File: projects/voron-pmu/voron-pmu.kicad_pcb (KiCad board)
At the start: 2 copper layers, 131 x 64.5 mm, 13 parts, among them J1 Critical loads, J2 Non-critical loads, J3 Critical supply, J4 Non-critical supply, J5 Pwr-loss-1, J6 Pwr-loss-2, K1 FINDER-40.52, K2 FINDER-40.52, K3 FINDER-40.52, K4 FINDER-40.52, SW1 SW_Push, SW2 SW_Push_Open

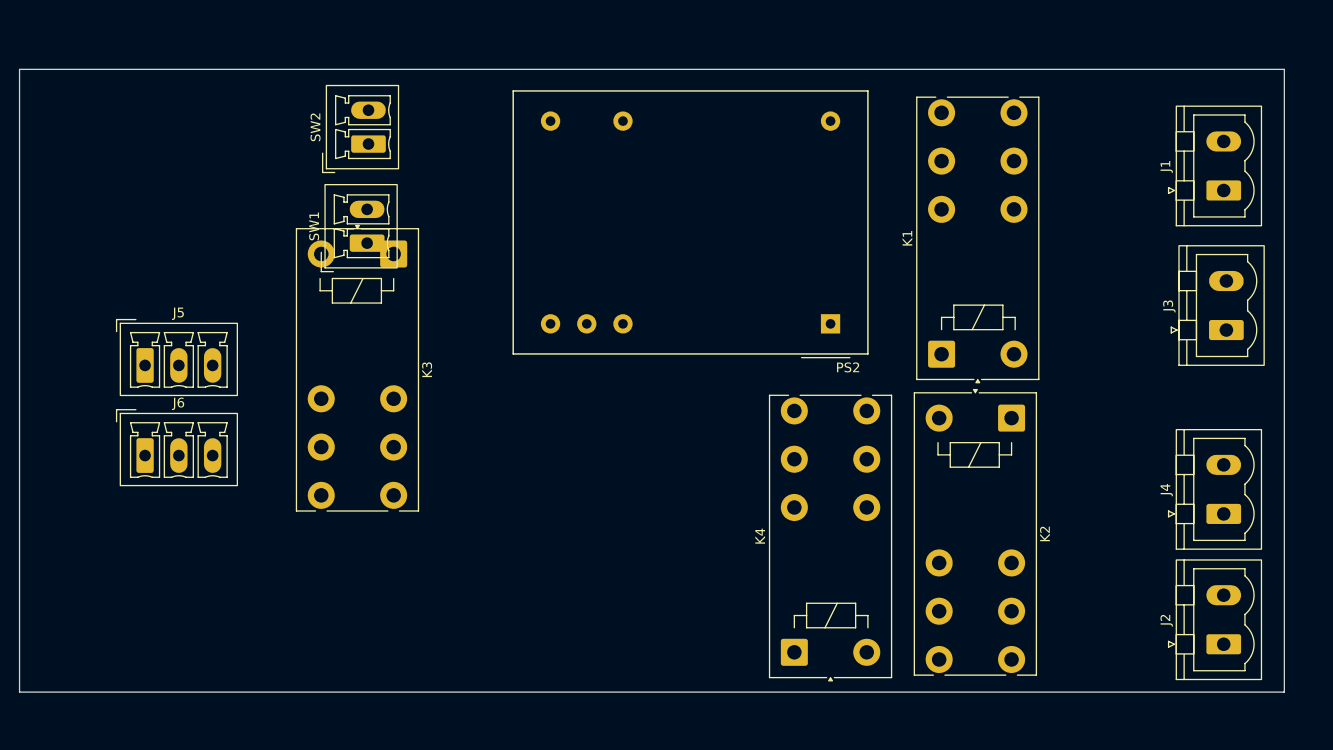
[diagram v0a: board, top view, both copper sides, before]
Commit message: Re-saving.
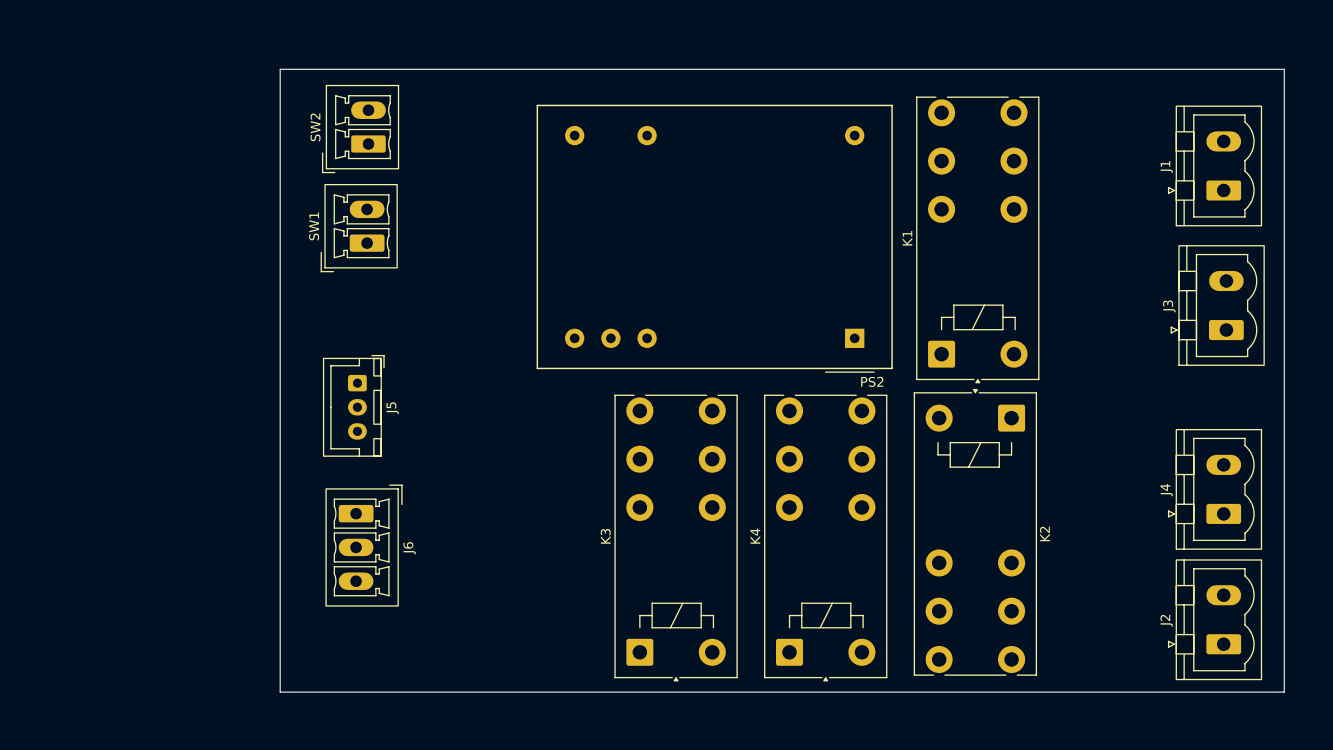
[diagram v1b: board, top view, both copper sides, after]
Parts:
- J5: footprint Connector_Phoenix_MC:PhoenixContact_MCV_1,5_3-G-3.5_1x03_P3.50mm_Vertical -> Connector_JST:JST_XH_B3B-XH-A_1x03_P2.50mm_Vertical
- moved K3 48.5 mm to (133.8, 110.4), turned to 90 degrees
- moved J6 22.7 mm to (104.4, 96.0), turned to -90 degrees
- moved J5 22.1 mm to (104.5, 82.5), turned to -90 degrees
- moved PS2 2.92 mm to (156.0, 77.9)
- moved K4 0.50 mm to (149.2, 110.4)
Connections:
- PS2 pad 5: unconnected-(PS2-AC(L)-Pad5) -> Net-(J3-Pin_1)
- PS2 pad 6: unconnected-(PS2-AC(N)-Pad6) -> Net-(J3-Pin_2)
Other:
- board size 131 x 64.5 mm -> 104 x 64.5 mm

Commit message: Prettyfing schematics.
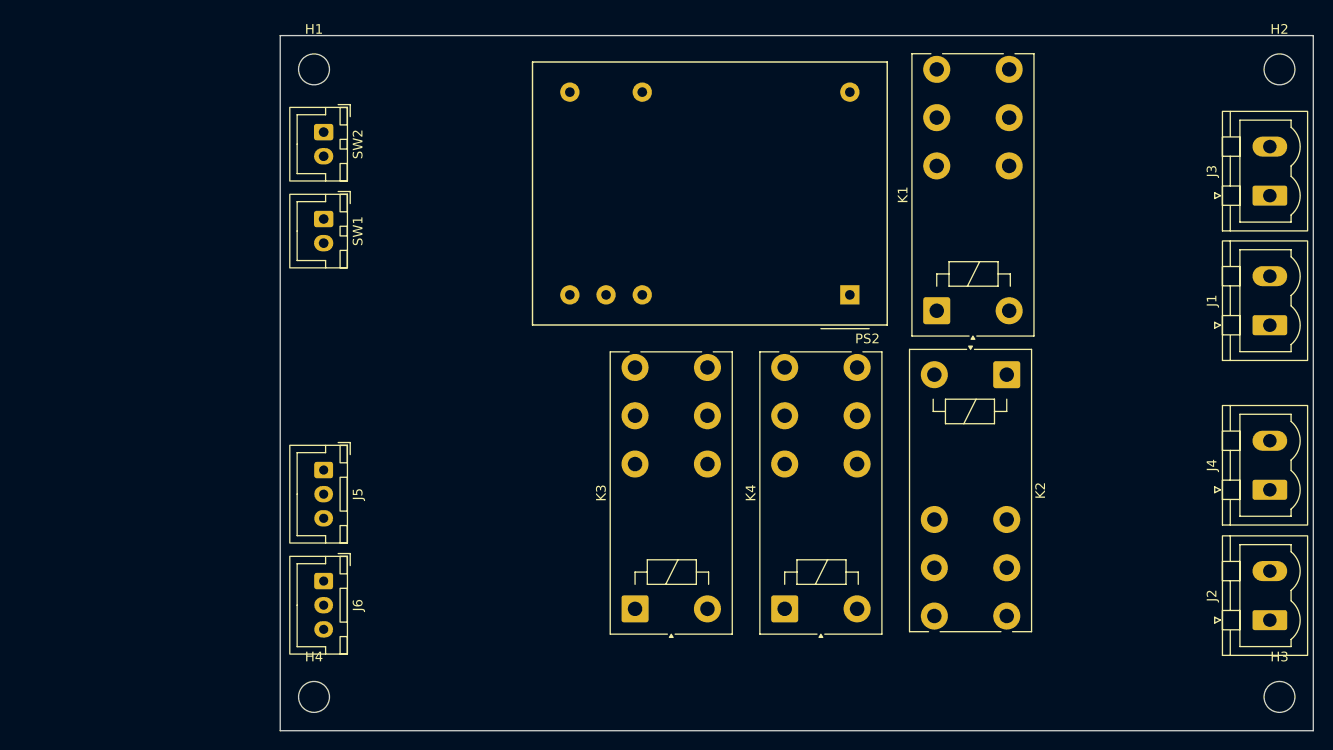
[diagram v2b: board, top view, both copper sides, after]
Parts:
- added H1: MountingHole, MountingHole:MountingHole_3.2mm_M3, F.Cu at (100.0, 50.0)
- added H2: MountingHole, MountingHole:MountingHole_3.2mm_M3, F.Cu at (200.0, 50.0)
- added H3: MountingHole, MountingHole:MountingHole_3.2mm_M3, F.Cu at (200.0, 115.0)
- added H4: MountingHole, MountingHole:MountingHole_3.2mm_M3, F.Cu at (100.0, 115.0)
- J6: footprint Connector_Phoenix_MC:PhoenixContact_MCV_1,5_3-G-3.5_1x03_P3.50mm_Vertical -> Connector_JST:JST_XH_B3B-XH-A_1x03_P2.50mm_Vertical
- SW1: value SW_Push -> sw-on; footprint Connector_Phoenix_MC:PhoenixContact_MCV_1,5_2-G-3.5_1x02_P3.50mm_Vertical -> Connector_JST:JST_XH_B2B-XH-A_1x02_P2.50mm_Vertical
- SW2: value SW_Push_Open -> sw-off; footprint Connector_Phoenix_MC:PhoenixContact_MCV_1,5_2-G-3.5_1x02_P3.50mm_Vertical -> Connector_JST:JST_XH_B2B-XH-A_1x02_P2.50mm_Vertical
- moved J1 14.8 mm to (199.0, 76.5)
- moved J3 14.6 mm to (199.0, 63.1)
- moved J5 9.66 mm to (101.0, 91.5)
- moved J6 7.75 mm to (101.0, 103.0)
- moved J2 5.39 mm to (199.0, 107.0)
- moved J4 5.39 mm to (199.0, 93.5)
- moved SW1 5.15 mm to (101.0, 65.5), turned to -90 degrees
- moved SW2 4.80 mm to (101.0, 56.5), turned to -90 degrees
- moved K1 4.53 mm to (164.5, 75.0)
- moved K2 4.53 mm to (171.8, 81.6)
- moved K3 4.53 mm to (133.2, 105.9)
- moved K4 4.53 mm to (148.8, 105.9)
- moved PS2 4.53 mm to (155.5, 73.4)
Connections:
- net power-good renamed +24V-sw
- PS2 pad 5: Net-(J3-Pin_1) -> Net-(J3-Pin_2)
- PS2 pad 6: Net-(J3-Pin_2) -> Net-(J3-Pin_1)
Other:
- board size 104 x 64.5 mm -> 107 x 72 mm
